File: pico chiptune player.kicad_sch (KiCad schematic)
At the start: 84 parts, among them J1 USB_C_5V3A, J2 MicroSD, J3 Speaker_L, J4 Speaker_R, Q1 AO3401A, Q2 2N7002, SW1 Play / Pause, SW2 Next, SW3 Previous, SW4 BOOTSEL, SW5 RESET, U1 YM2149F, U2 0.96"OLED_I2C, U3 PAM8403, U4 YM2149F, U5 RP2354A, U6 AMS1117-3.3, U8 74HCT4053D, U9 74HCT4053D, Y1 12MHz

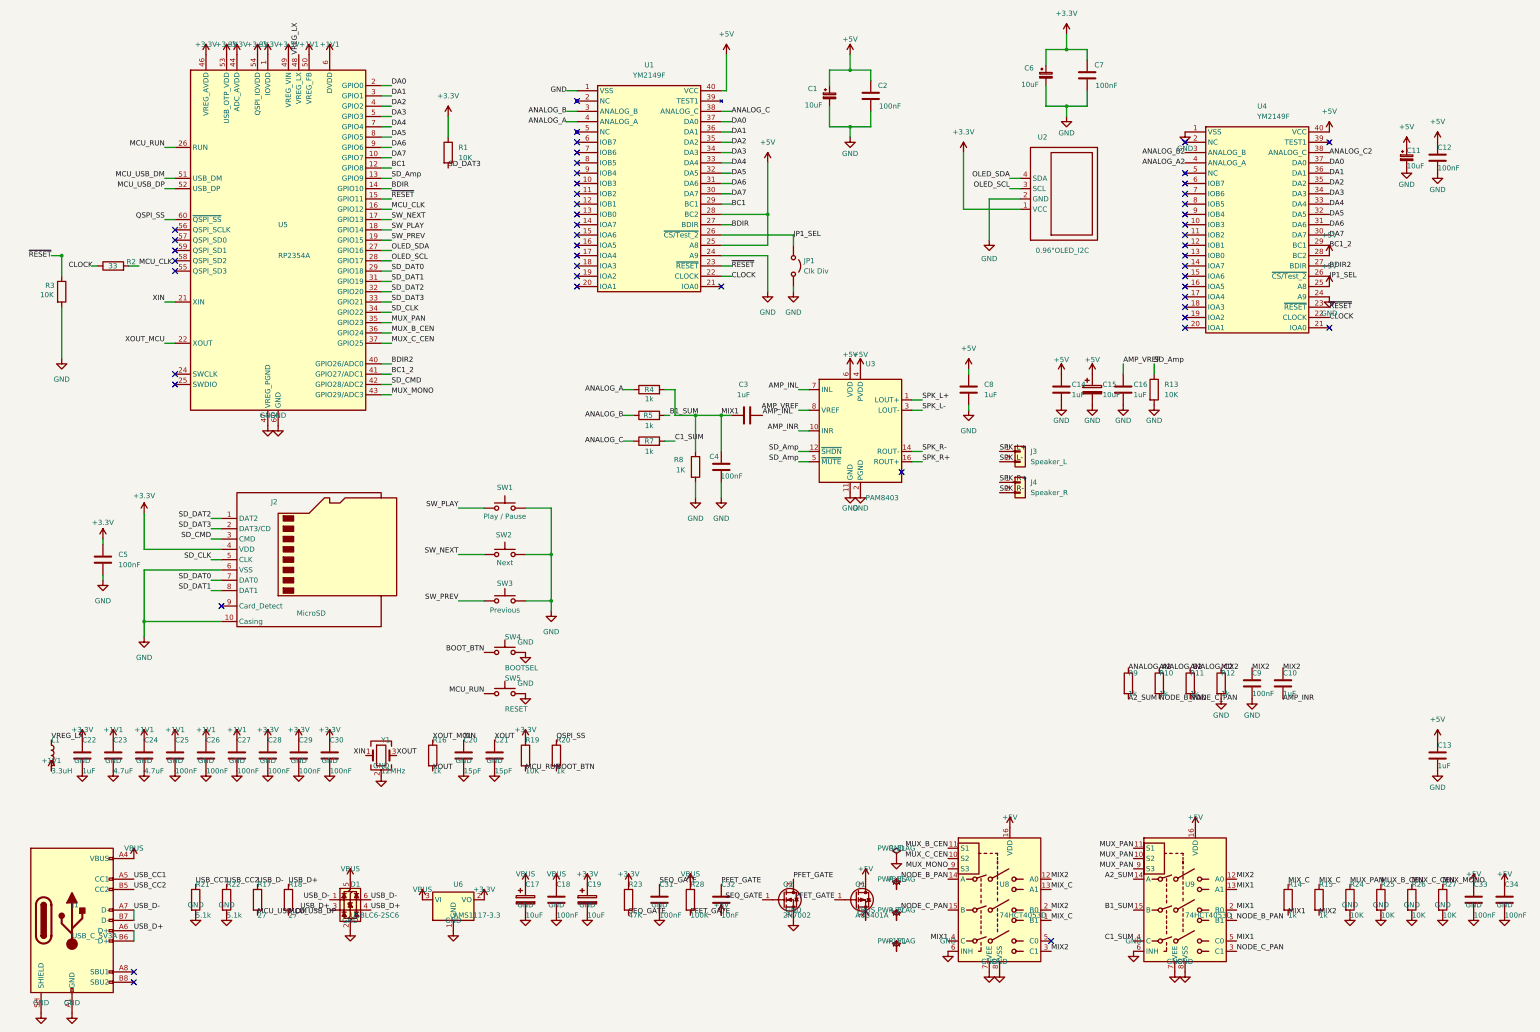
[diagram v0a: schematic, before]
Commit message: Implement code changes to enhance functionality and improve performance
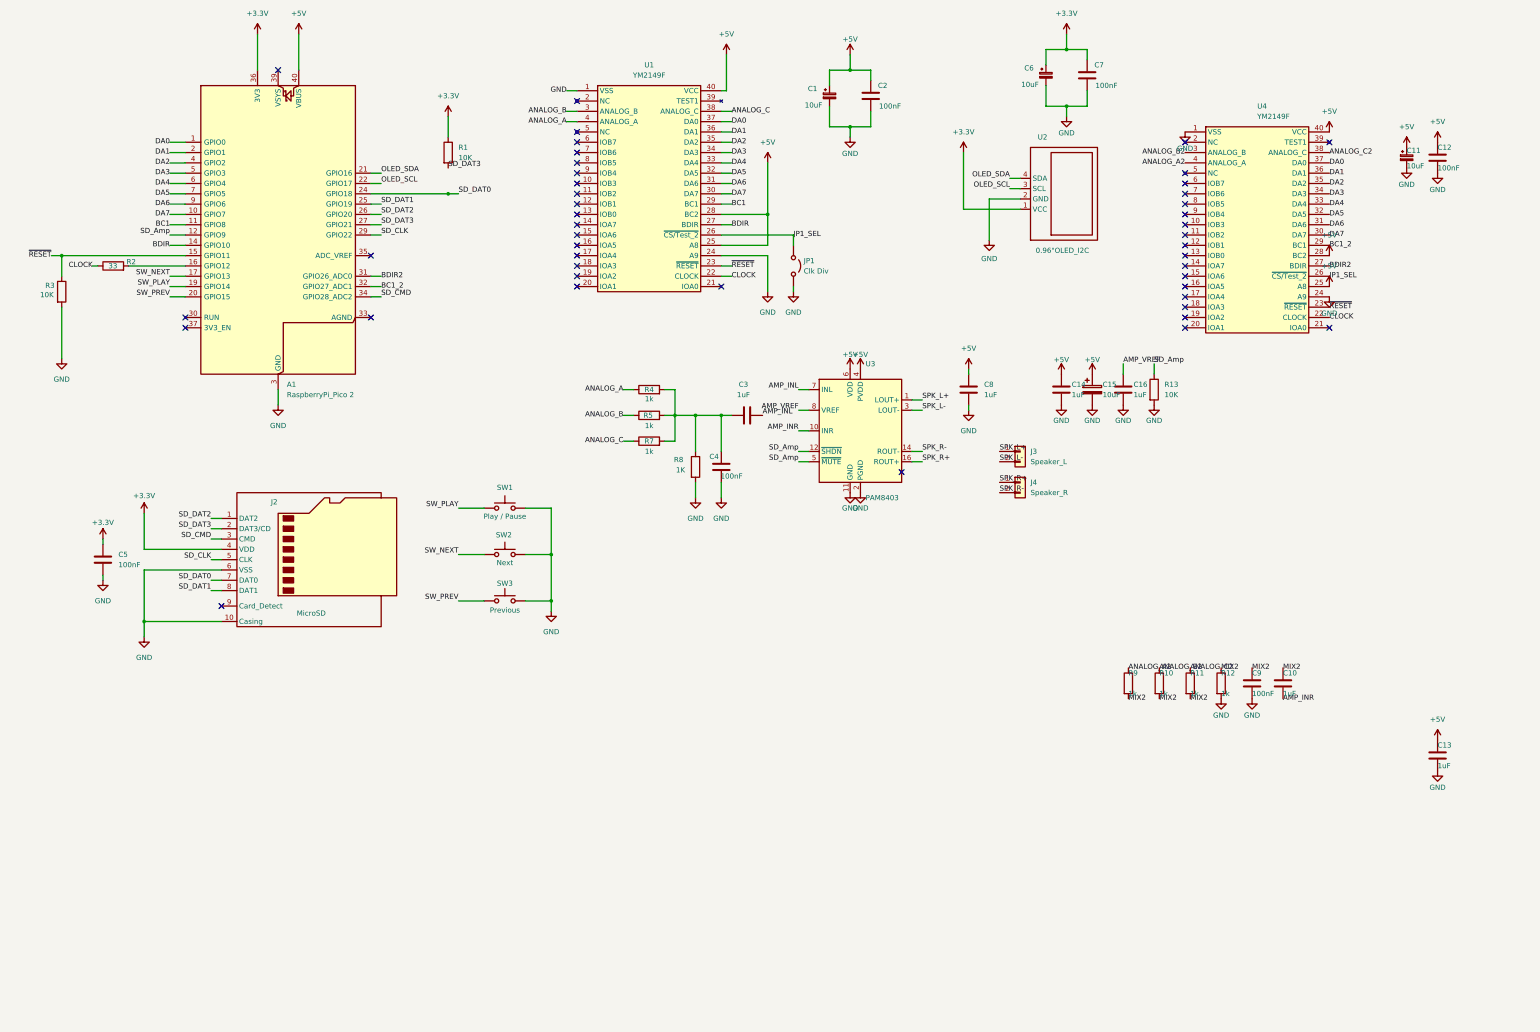
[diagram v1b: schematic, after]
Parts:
- removed C17, C19: 10uF, Capacitor_SMD:CP_Elec_4x5.4, symbol Device:C_Polarized
- removed C18, C25, C26, C27, C28, C29, C30, C31, C33, C34: 100nF, Capacitor_SMD:C_0805_2012Metric_Pad1.18x1.45mm_HandSolder, symbol Device:C
- removed C20, C21: 15pF, Capacitor_SMD:C_0805_2012Metric_Pad1.18x1.45mm_HandSolder, symbol Device:C
- removed C22: 1uF, Capacitor_SMD:C_0805_2012Metric_Pad1.18x1.45mm_HandSolder, symbol Device:C
- removed C23, C24: 4.7uF, Capacitor_SMD:C_0805_2012Metric_Pad1.18x1.45mm_HandSolder, symbol Device:C
- removed C32: 10nF, Capacitor_SMD:C_0805_2012Metric_Pad1.18x1.45mm_HandSolder, symbol Device:C
- removed D1: USBLC6-2SC6, Package_TO_SOT_SMD:SOT-23-6, symbol Power_Protection:USBLC6-2SC6
- removed J1: USB_C_5V3A, Connector_USB:USB_C_Receptacle_HRO_TYPE-C-31-M-12, symbol Connector:USB_C_Receptacle_USB2.0_16P
- removed L1: 3.3uH, Inductor_SMD:L_1210_3225Metric, symbol Device:L
- removed Q1: AO3401A, Package_TO_SOT_SMD:SOT-23, symbol Transistor_FET:AO3401A
- removed Q2: 2N7002, Package_TO_SOT_SMD:SOT-23, symbol Transistor_FET:2N7002
- removed R14, R15, R16, R20: 1k, Resistor_SMD:R_0805_2012Metric_Pad1.20x1.40mm_HandSolder, symbol Device:R
- removed R17, R18: 27, Resistor_SMD:R_0805_2012Metric_Pad1.20x1.40mm_HandSolder, symbol Device:R
- removed R19, R24, R25, R26, R27: 10K, Resistor_SMD:R_0805_2012Metric_Pad1.20x1.40mm_HandSolder, symbol Device:R
- removed R21, R22: 5.1k, Resistor_SMD:R_0805_2012Metric_Pad1.20x1.40mm_HandSolder, symbol Device:R
- removed R23: 47K, Resistor_SMD:R_0805_2012Metric_Pad1.20x1.40mm_HandSolder, symbol Device:R
- removed R28: 100K, Resistor_SMD:R_0805_2012Metric_Pad1.20x1.40mm_HandSolder, symbol Device:R
- removed SW4: BOOTSEL, Button_Switch_THT:SW_PUSH_6mm, symbol Switch:SW_Push
- removed SW5: RESET, Button_Switch_THT:SW_PUSH_6mm, symbol Switch:SW_Push
- removed U5: RP2354A, Package_DFN_QFN:QFN-60-1EP_7x7mm_P0.4mm_EP3.4x3.4mm, symbol MCU_RaspberryPi:RP2354A
- removed U6: AMS1117-3.3, Package_TO_SOT_SMD:SOT-223-3_TabPin2, symbol Regulator_Linear:AMS1117-3.3
- removed U8, U9: 74HCT4053D, Package_SO:SOIC-16_3.9x9.9mm_P1.27mm, symbol Analog_Switch:CD4053B
- removed Y1: 12MHz, Crystal:Crystal_SMD_3225-4Pin_3.2x2.5mm, symbol Device:Crystal_GND24
- added A1: RaspberryPi_Pico 2, TMCu Module:RPi_Pico_SMD_TH, symbol MCU_Module_RaspberryPi_Pico:RaspberryPi_Pico
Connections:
- net A2_SUM is gone; now on net MIX2: R9.2
- net C1_SUM is gone; now on an unnamed net: R7.2
- net MIX1 is gone; now on an unnamed net: C3.1, C4.1, R4.2, R8.1
- net NODE_B_PAN is gone; now on net MIX2: R10.2
- net NODE_C_PAN is gone; now on net MIX2: R11.2
- net +3.3V: now also A1.36 (3V3)
- net +5V: now also A1.40 (VBUS)
- net BC1: now also A1.11 (GPIO8)
- net BC1_2: now also A1.32 (GPIO27_ADC1)
- net BDIR: now also A1.14 (GPIO10)
- net BDIR2: now also A1.31 (GPIO26_ADC0)
- net DA0: now also A1.1 (GPIO0)
- net DA1: now also A1.2 (GPIO1)
- net DA2: now also A1.4 (GPIO2)
- net DA3: now also A1.5 (GPIO3)
- net DA4: now also A1.6 (GPIO4)
- net DA5: now also A1.7 (GPIO5)
- net DA6: now also A1.9 (GPIO6)
- net DA7: now also A1.10 (GPIO7)
- net GND: now also A1.13 (GND), A1.18 (GND), A1.23 (GND), A1.28 (GND), A1.3 (GND), A1.38 (GND), A1.8 (GND)
- net OLED_SCL: now also A1.22 (GPIO17)
- net OLED_SDA: now also A1.21 (GPIO16)
- net SD_Amp: now also A1.12 (GPIO9)
- net SD_CLK: now also A1.29 (GPIO22)
- net SD_CMD: now also A1.34 (GPIO28_ADC2)
- net SD_DAT0: now also A1.24 (GPIO18)
- net SD_DAT1: now also A1.25 (GPIO19)
- net SD_DAT2: now also A1.26 (GPIO20)
- net SD_DAT3: now also A1.27 (GPIO21)
- net SW_NEXT: now also A1.17 (GPIO13)
- net SW_PLAY: now also A1.19 (GPIO14)
- net SW_PREV: now also A1.20 (GPIO15)
- net ~{RESET}: now also A1.15 (GPIO11)
- net B1_SUM: no longer names the net of R5.2
- net MCU_CLK: no longer names the net of R2.2
- net MCU_CLK: now also A1.16 (GPIO12)
- no-connect marks 49 -> 44
